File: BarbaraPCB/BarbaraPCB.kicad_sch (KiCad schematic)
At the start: 138 parts, among them J1 Conn_01x05_Pin, J2 Conn_01x05_Pin, J3 Conn_01x05_Pin_reversed, J4 Conn_01x05_Pin_reversed, SW1 SW_Push, SW10 SW_Push, SW11 SW_Push, SW12 SW_Push, SW13 SW_Push, SW14 SW_Push, SW15 SW_Push, SW16 SW_Push, SW17 SW_Push, SW18 SW_Push, SW19 SW_Push, SW2 SW_Push, SW20 SW_Push, SW21 SW_Push_1.5u, SW22 SW_Push, SW23 SW_Push, SW24 SW_Push, SW25 SW_Push, SW26 SW_Push, SW27 SW_Push, SW28 SW_Push, SW29 SW_Push_1.5u, SW3 SW_Push, SW30 SW_Push, SW31 SW_Push, SW32 SW_Push, SW33 SW_Push, SW34 SW_Push, SW35 SW_Push_1.25u, SW36 SW_Push_1.75u, SW37 SW_Push_1.75u, SW38 SW_Push_1.25u, SW39 SW_Push, SW4 SW_Push, SW40 SW_Push, SW41 SW_Push, SW42 SW_Push, SW43 SW_Push, SW44 SW_Push, SW45 SW_Push_1.5u, SW46 SW_Push_1.5u, SW47 SW_Push_1.5u, SW48 SW_Push_1.5u, SW49 SW_Push, SW5 SW_Push, SW50 SW_Push, SW51 SW_Push, SW52 SW_Push, SW53 SW_Push, SW54 SW_Push_1.25u, SW55 SW_Push_1.75u, SW56 SW_Push_1.75u, SW57 SW_Push_1.25u, SW58 SW_Push, SW59 SW_Push, SW6 SW_Push, SW60 SW_Push, SW61 SW_Push, SW62 SW_Push, SW63 SW_Push, SW64 SW_Push_1.5u, SW65 SW_Push_1.5u, SW66 SW_Push_1.5u, SW67 SW_Push_1.5u, SW7 SW_Push, SW8 SW_Push, SW9 SW_Push

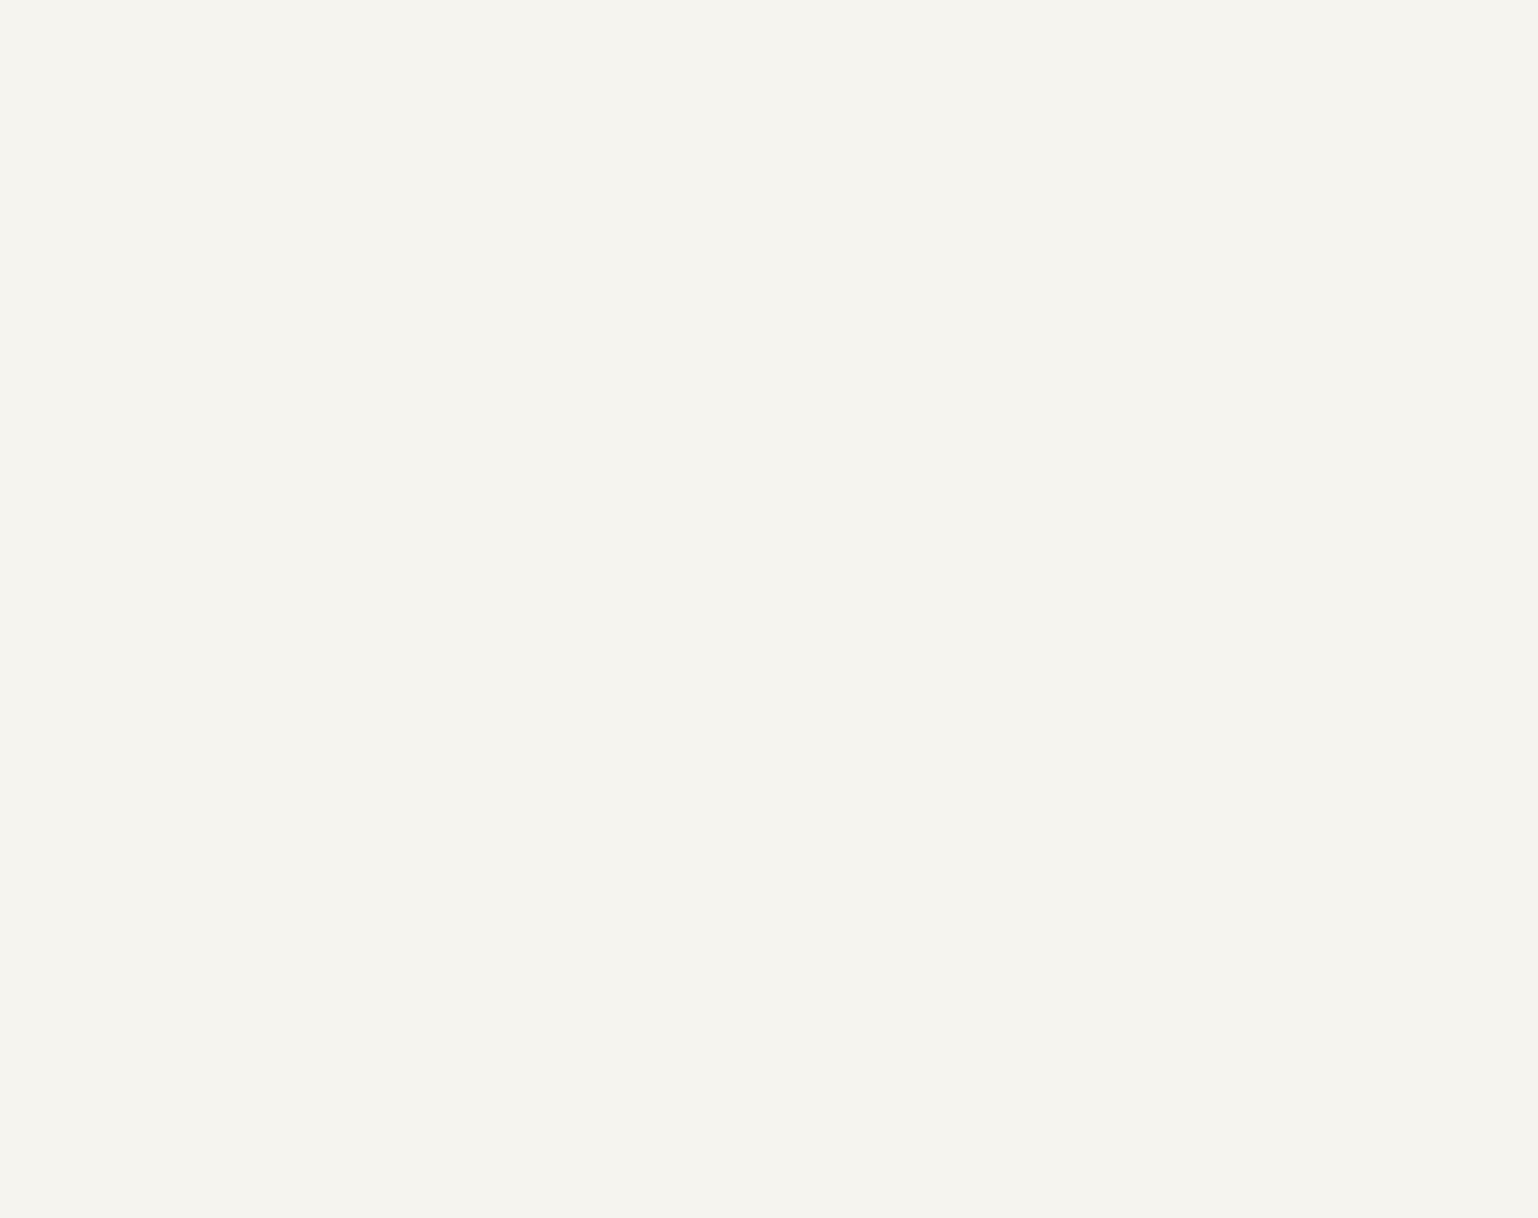
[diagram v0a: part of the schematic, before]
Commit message: Soundbauteile hinzugefügt
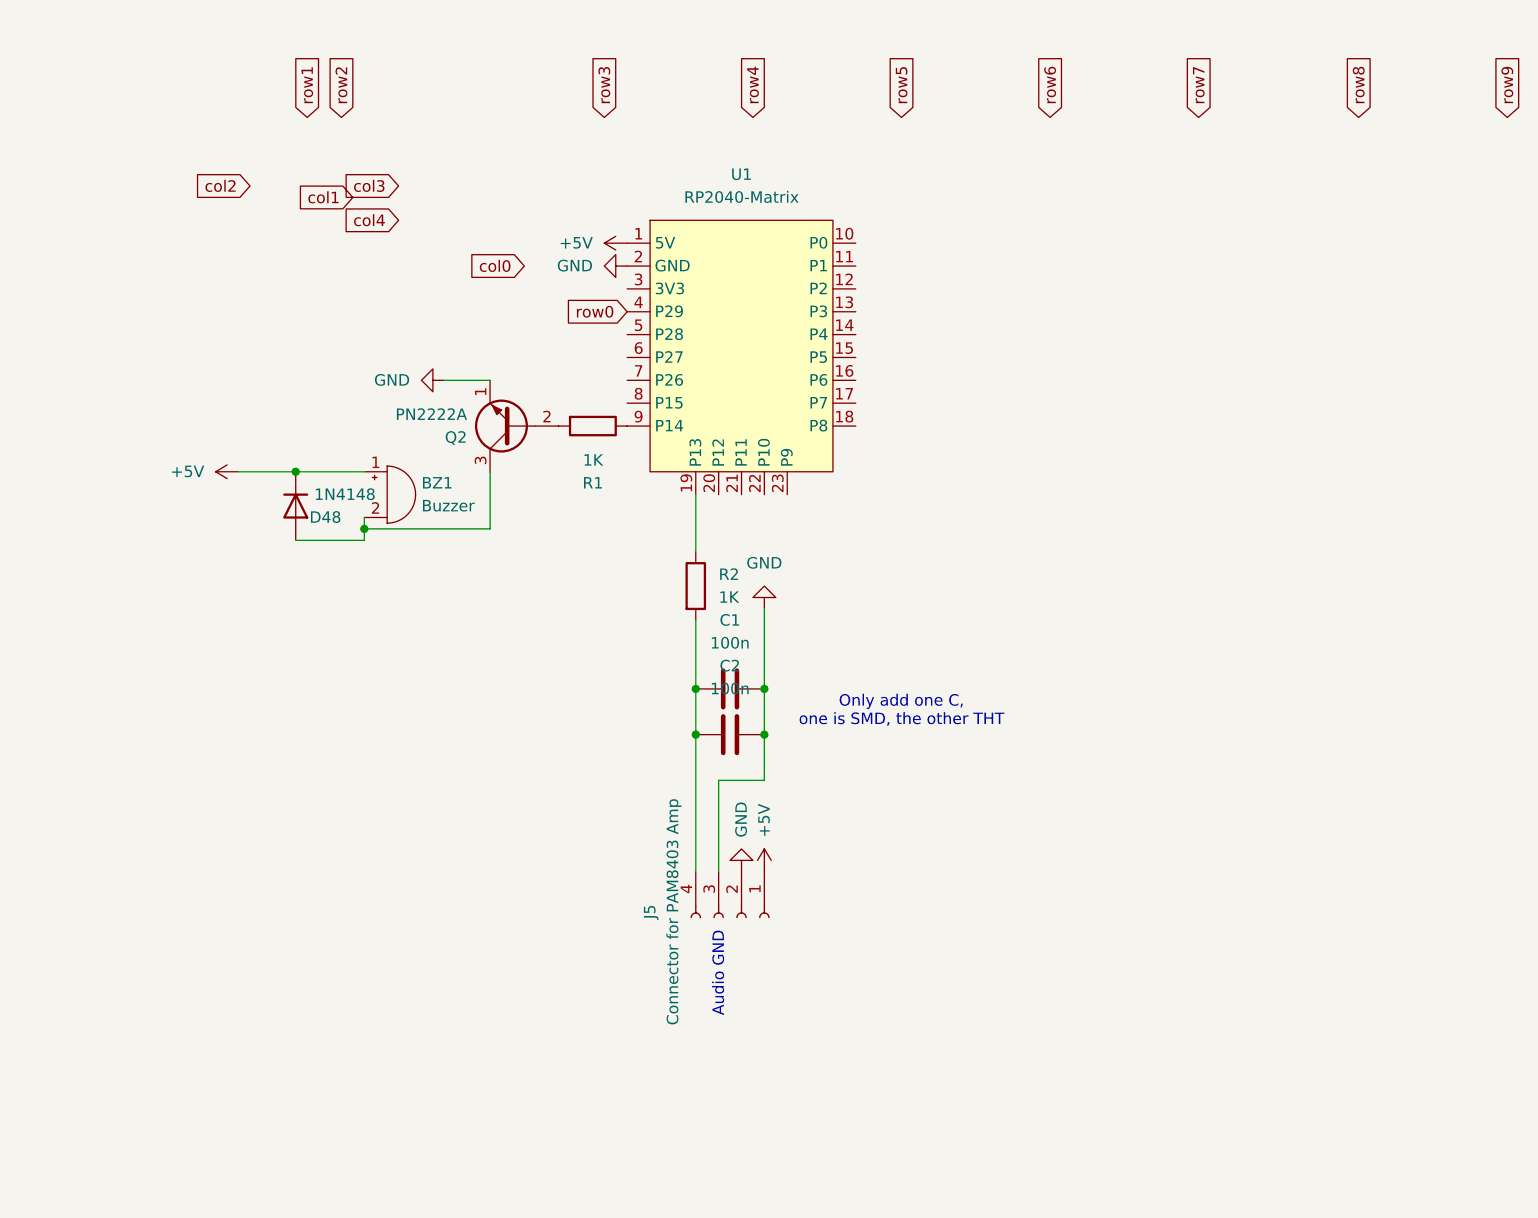
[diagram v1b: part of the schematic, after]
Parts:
- added BZ1: Buzzer, Buzzer_Beeper:MagneticBuzzer_StarMicronics_QMB-105, symbol Device:Buzzer
- added C1: 100n, Capacitor_THT:C_Disc_D5.0mm_W2.5mm_P5.00mm, symbol Device:C
- added C2: 100n, Capacitor_SMD:C_0805_2012Metric_Pad1.18x1.45mm_HandSolder, symbol Device:C
- added D48: 1N4148, TFL:Diode-dual, symbol Diode:1N4148
- added J5: Connector for PAM8403 Amp, Connector_PinHeader_2.54mm:PinHeader_1x04_P2.54mm_Vertical, symbol Connector:Conn_01x04_Socket
- added Q2: PN2222A, Package_TO_SOT_THT:TO-92_Inline, symbol Transistor_BJT:PN2222A
- added R1, R2: 1K, TFL:Diode-dual, symbol Device:R
- added U1: RP2040-Matrix, TFL:RP2040-Gemini-BigHole, symbol PCM_marbastlib-promicroish:RP2040-Matrix
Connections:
- net row0: now also U1.4 (P29)
- new net: C1.1, C2.1, J5.4 (Pin_4), R2.2
- new net: R2.1, U1.19 (P13)
- new net: R1.1, U1.9 (P14)
- new net: BZ1.2 (-), D48.2 (A), Q2.3 (C)
- new net: Q2.2 (B), R1.2
- new net +5V: BZ1.1 (+), D48.1 (K), J5.1 (Pin_1), U1.1 (5V)
- new net GND: C1.2, C2.2, J5.2 (Pin_2), J5.3 (Pin_3), Q2.1 (E), U1.2 (GND)
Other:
- note added: "Audio GND"
- note added: "Only add one C, one is SMD, the other THT"
